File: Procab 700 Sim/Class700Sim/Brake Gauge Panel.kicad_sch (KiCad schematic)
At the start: 24 parts, among them SW29 SW-EMG, SW30 SW-DRA, SW31 SW-PCB, SW36 SW-DSKL, SW37 SW-WSH, SW38 SW-WSW, SW39 SWAWS, SW40 SWAWS, SW41 SWAWS, SW42 SWAWS, SW43 SWAWS, SW44 SWAWS, SW45 SWAWS, SW46 SWAWS, SW47 SWAWS, SW48 SWAWS, SW49 SWAWS, SW50 SWAWS, SW51 SWAWS, SW52 SWAWS

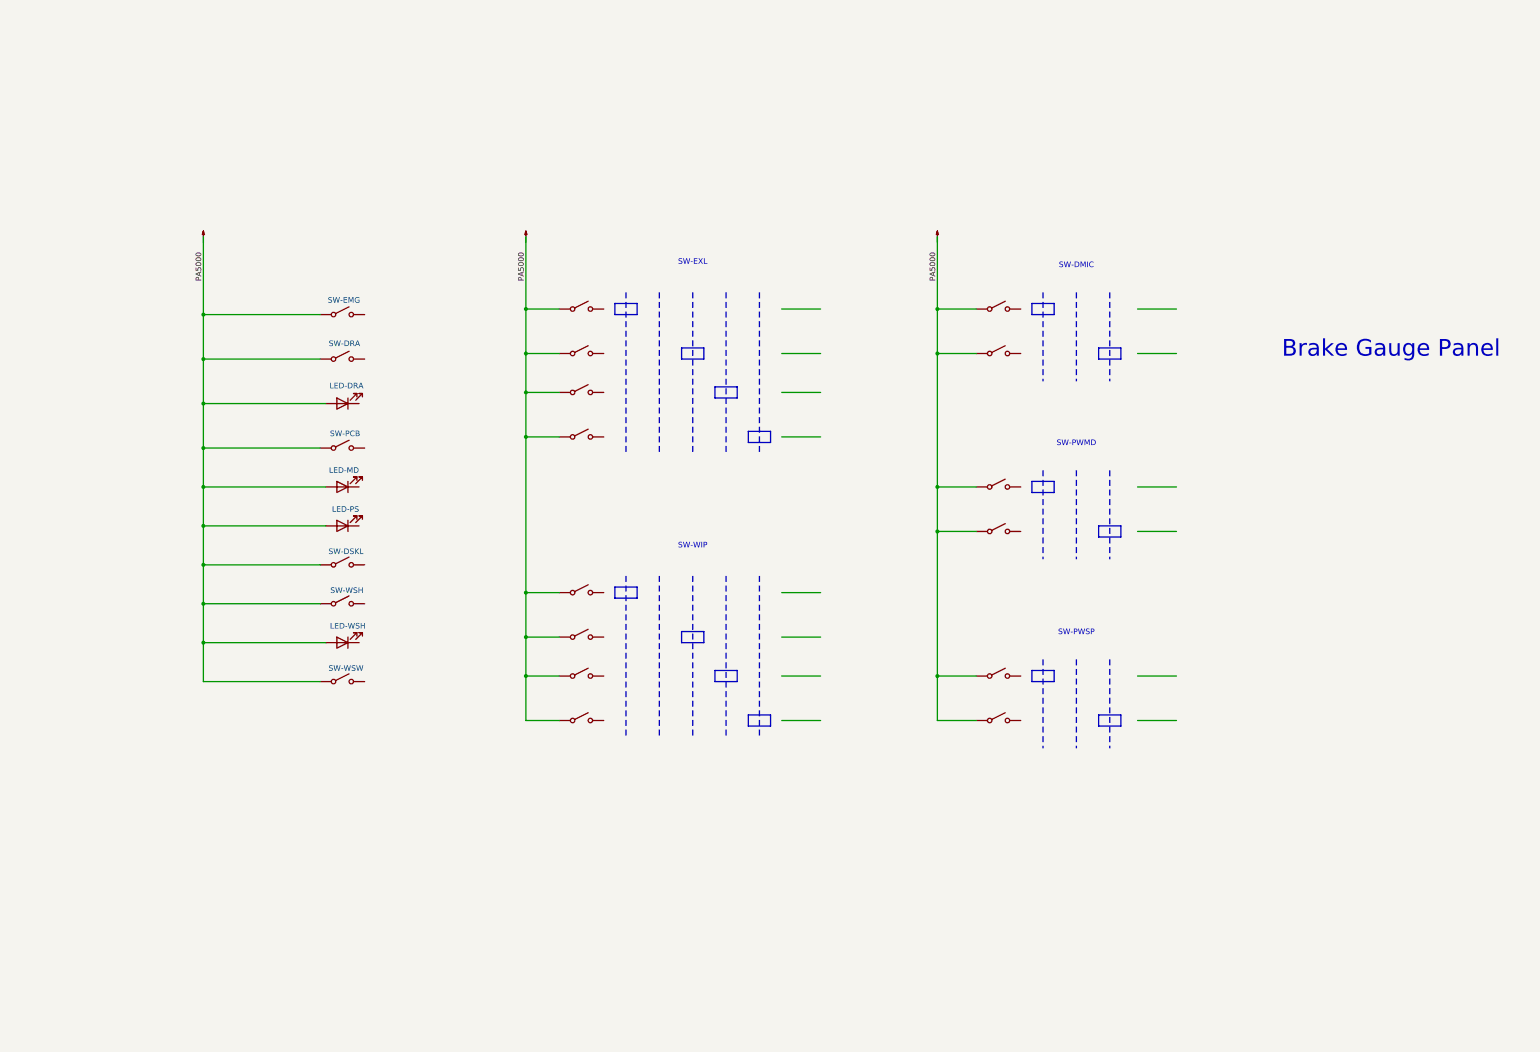
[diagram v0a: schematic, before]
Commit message: Changes made
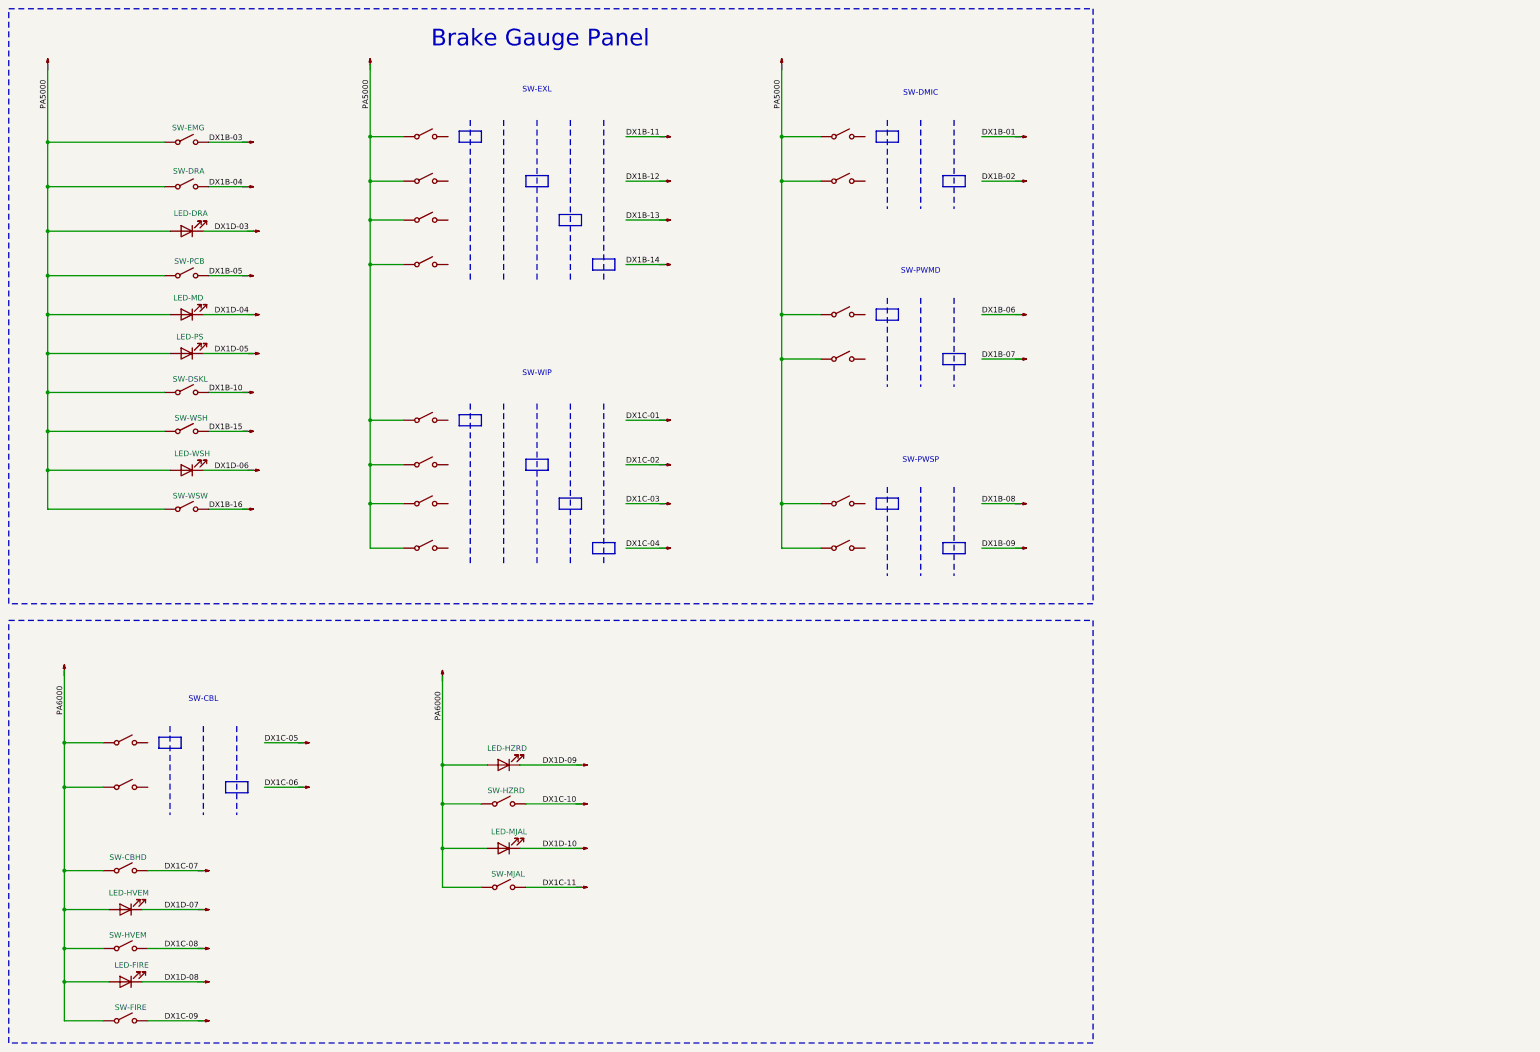
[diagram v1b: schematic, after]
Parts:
- added D10: LED-HZRD, symbol Device:LED
- added D11: LED-MJAL, symbol Device:LED
- added D4: LED-HVEM, symbol Device:LED
- added D9: LED-FIRE, symbol Device:LED
- added SW22: SW-CBHD, symbol Switch:SW_SPST
- added SW23: SW-FIRE, symbol Switch:SW_SPST
- added SW24: SW-HZRD, symbol Switch:SW_SPST
- added SW25: SW-MJAL, symbol Switch:SW_SPST
- added SW7, SW8: SWAWS, symbol Switch:SW_SPST
- added SW9: SW-HVEM, symbol Switch:SW_SPST
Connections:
- net DX1D-04: now reaches D6.1 (K)
- net DX1D-06: now reaches D8.1 (K)
- net DX1D-03: now reaches D5.1 (K)
- net DX1D-05: now reaches D7.1 (K)
- new net DX1B-03: SW29. (B)
- new net DX1B-04: SW30. (B)
- new net DX1B-05: SW31. (B)
- new net DX1B-10: SW36. (B)
- new net DX1B-15: SW37. (B)
- new net DX1B-16: SW38. (B)
- new net DX1C-07: SW22. (B)
- new net DX1C-08: SW9. (B)
- new net DX1C-09: SW23. (B)
- new net DX1C-10: SW24. (B)
- new net DX1C-11: SW25. (B)
- new net DX1D-07: D4.1 (K)
- new net DX1D-08: D9.1 (K)
- new net DX1D-09: D10.1 (K)
- new net DX1D-10: D11.1 (K)
- new net PA6000: D10.2 (A), D11.2 (A), D4.2 (A), D9.2 (A), SW22. (B), SW23. (B), SW24. (B), SW25. (B), SW7. (B), SW8. (B), SW9. (B)
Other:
- note added: "SW-CBL"
